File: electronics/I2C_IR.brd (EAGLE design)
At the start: 11 x 15.9 mm, 10 parts

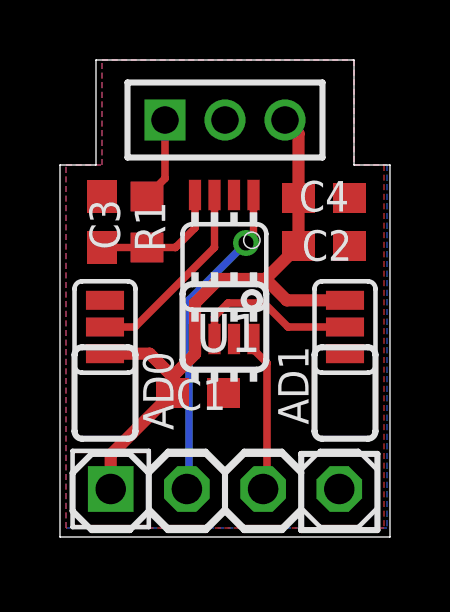
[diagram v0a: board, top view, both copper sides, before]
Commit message: Revised board layout
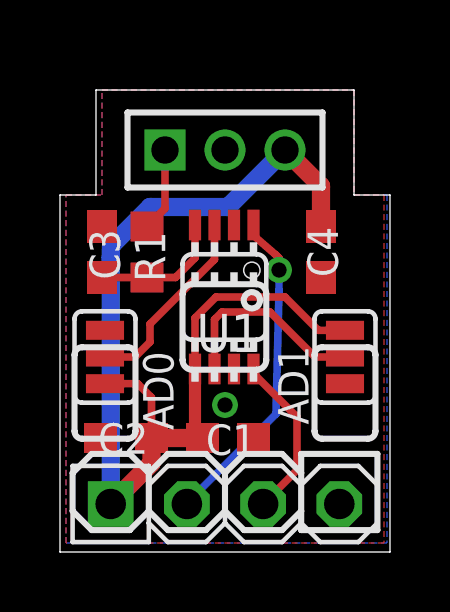
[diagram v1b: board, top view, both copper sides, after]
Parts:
- removed U$1: ADC081C021, mes_adc:MSOP8_0.65
- added U1: ADC081C021, mes_adc:MSOP8_0.65
- moved C2 9.19 mm to (2.20, 3.30), turned to 180 degrees
- moved C4 1.80 mm to (8.70, 9.50), turned to 270 degrees
- moved C1 1.80 mm to (5.60, 3.30)
- moved C3 1.00 mm to (1.40, 9.50)
- moved JP3 1.00 mm to (5.50, 12.9)
- moved R1 1.00 mm to (2.90, 9.50)
- moved SJ1 1.00 mm to (1.50, 6.00)
- moved SJ2 1.00 mm to (9.50, 6.00)
- moved JP1 0.50 mm to (5.50, 1.10)
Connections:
- net ADR0: now also U1.3; no longer U$1.3
- net ADR1: now also U1.6; no longer U$1.6
- net ALERT: now also U1.2; no longer U$1.2
- net GND: now also U1.7; no longer U$1.7
- net N$4: now also U1.4; no longer U$1.4
- net SCL: now also U1.1; no longer U$1.1
- net SDA: now also U1.8; no longer U$1.8
- net VCC: now also U1.5; no longer U$1.5
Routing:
- net VCC: track 21.5 -> 36.2 mm
- net ADR1: track 5.62 -> 6.72 mm
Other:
- board size 11 x 15.9 mm -> 11 x 15.4 mm
